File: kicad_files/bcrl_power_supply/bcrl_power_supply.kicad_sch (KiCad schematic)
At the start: 10 parts, among them J1 OSTVN02A150, J12 5034801600, J2 OSTVN02A150, J3 Conn_01x02

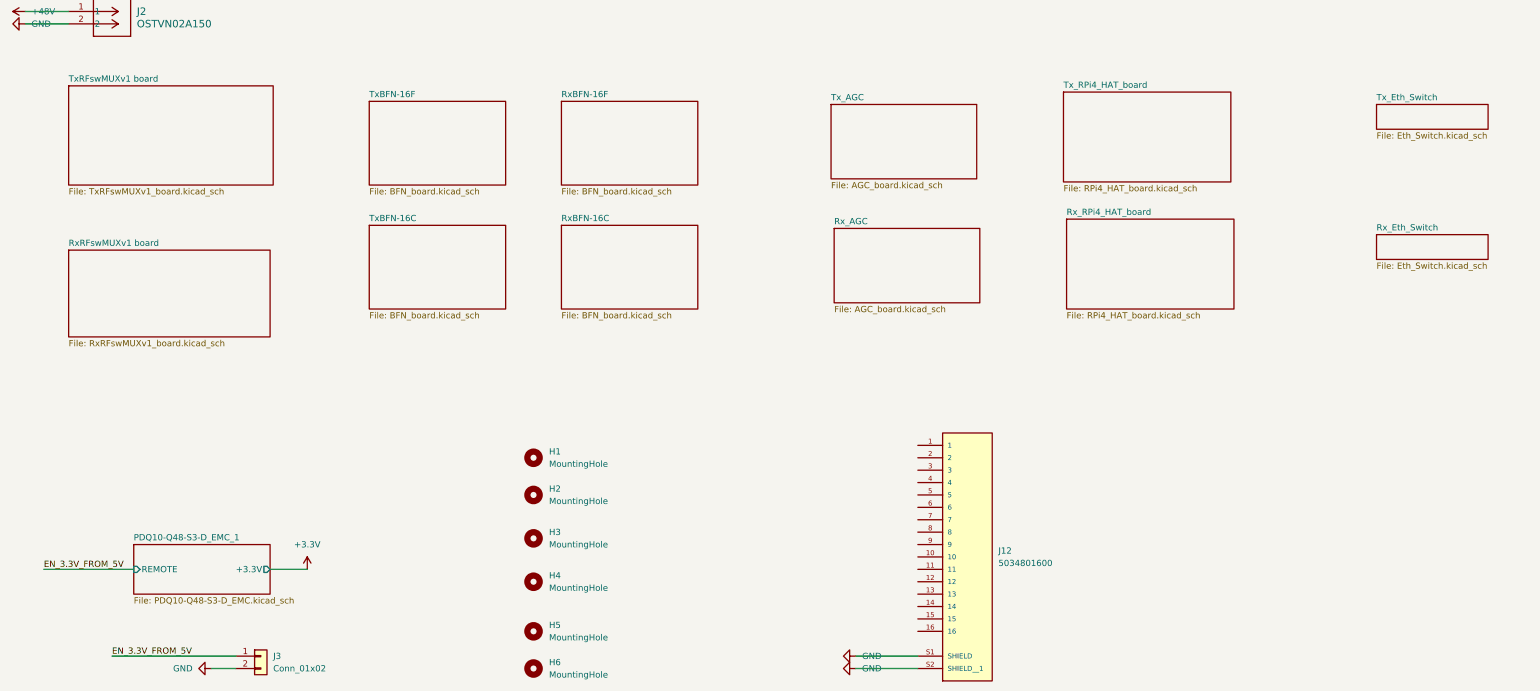
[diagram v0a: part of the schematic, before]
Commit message: almost done schematic
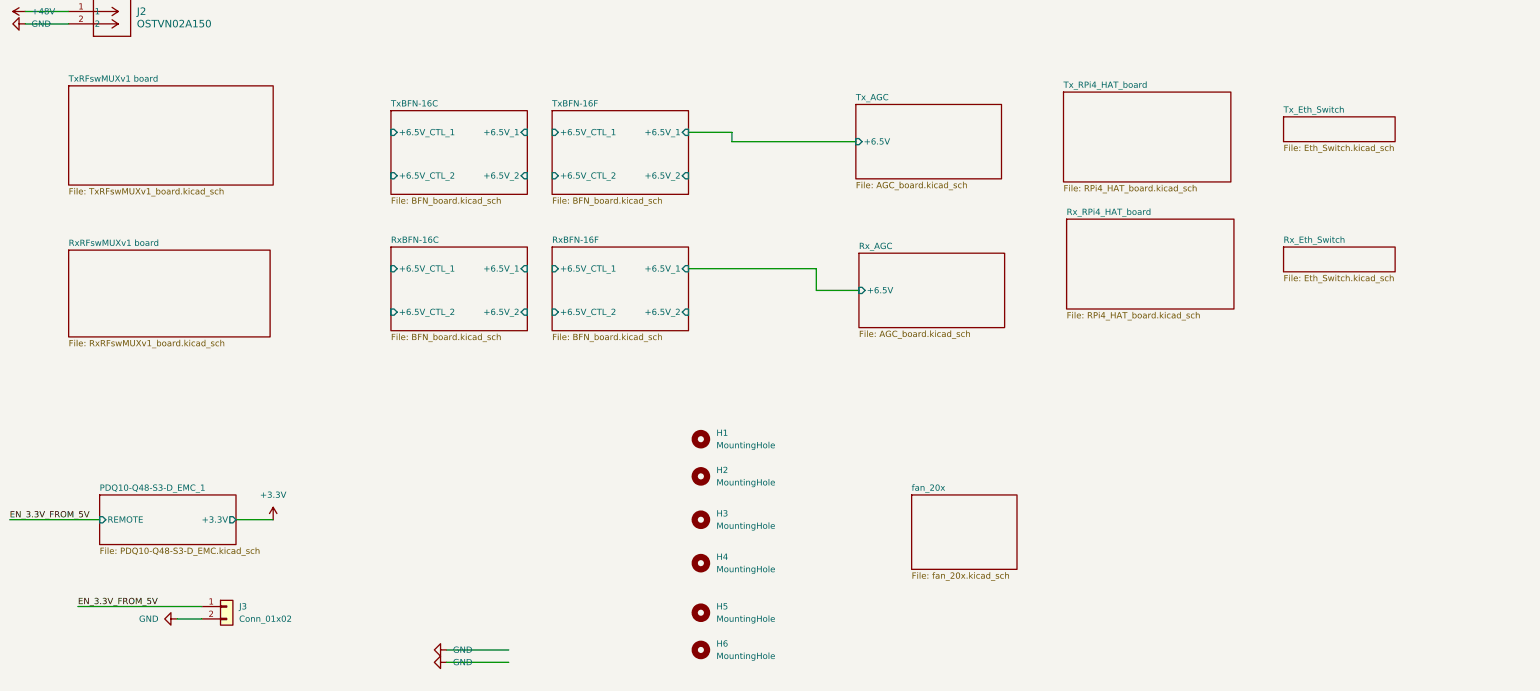
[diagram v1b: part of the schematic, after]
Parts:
- removed J12: 5034801600, BCRL_power_supply:MOLEX_5034801600, symbol BCRL_power_supply:5034801600
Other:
- added sheet fan_20x (fan_20x.kicad_sch)
- sheet RxBFN-16C ports: added +6.5V_1, +6.5V_2, +6.5V_CTL_1, +6.5V_CTL_2; removed none
- sheet RxBFN-16F ports: added +6.5V_1, +6.5V_2, +6.5V_CTL_1, +6.5V_CTL_2; removed none
- sheet Rx_AGC ports: added +6.5V; removed none
- sheet TxBFN-16C ports: added +6.5V_1, +6.5V_2, +6.5V_CTL_1, +6.5V_CTL_2; removed none
- sheet TxBFN-16F ports: added +6.5V_1, +6.5V_2, +6.5V_CTL_1, +6.5V_CTL_2; removed none
- sheet Tx_AGC ports: added +6.5V; removed none
- moved on the sheet: H1, H2, H3, H4, H5, H6, J3

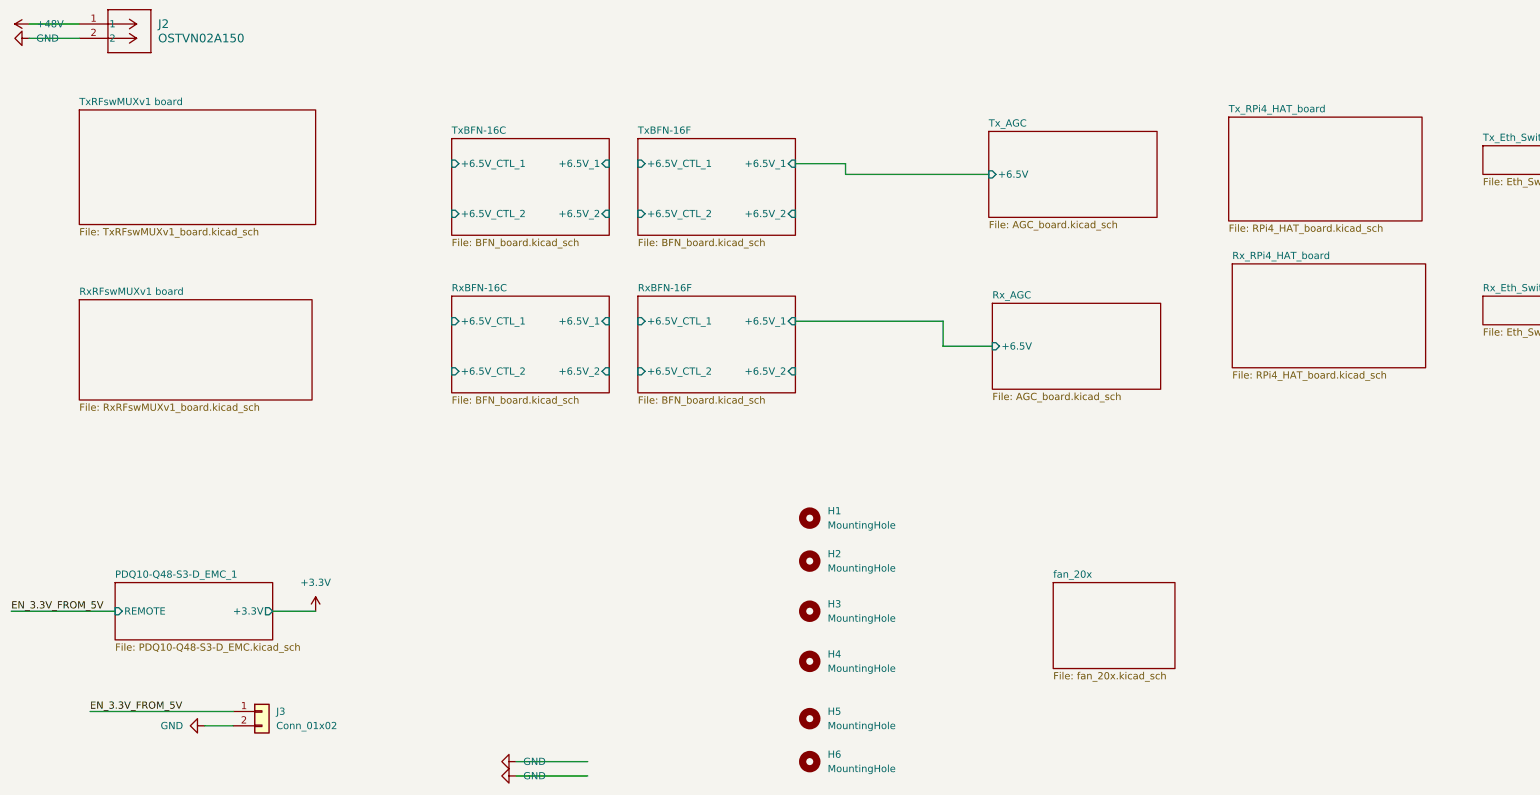
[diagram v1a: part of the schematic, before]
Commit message: schematic done
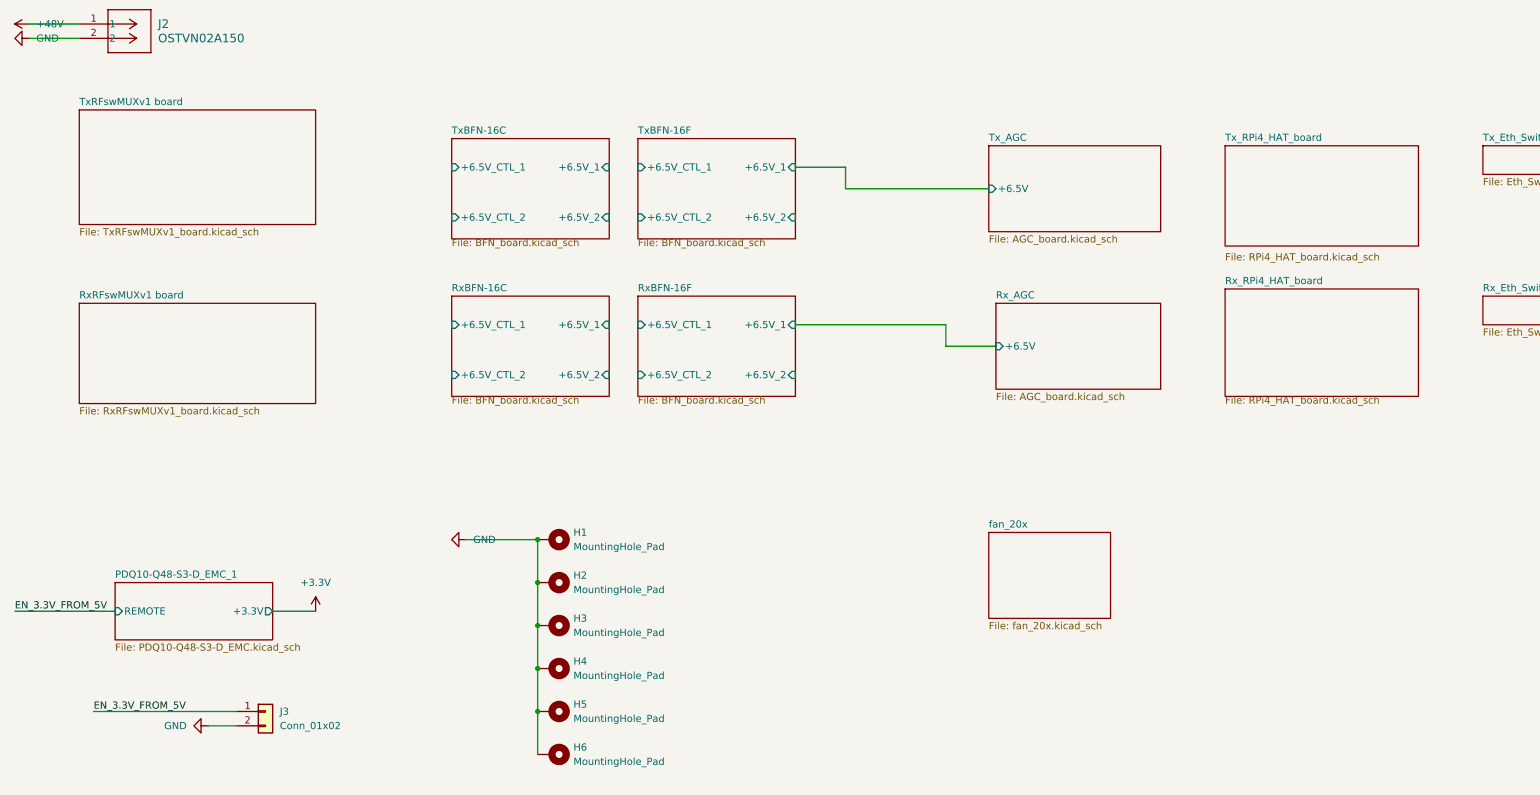
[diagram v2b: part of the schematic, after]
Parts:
- removed H1, H2, H3, H4, H5, H6: MountingHole, MountingHole:MountingHole_3.5mm_Pad, symbol Mechanical:MountingHole
- added H1, H2, H3, H4, H5, H6: MountingHole_Pad, MountingHole:MountingHole_3.5mm_Pad, symbol Mechanical:MountingHole_Pad
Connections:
- net GND: now also H1.1, H2.1, H3.1, H4.1, H5.1, H6.1
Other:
- moved on the sheet: J3

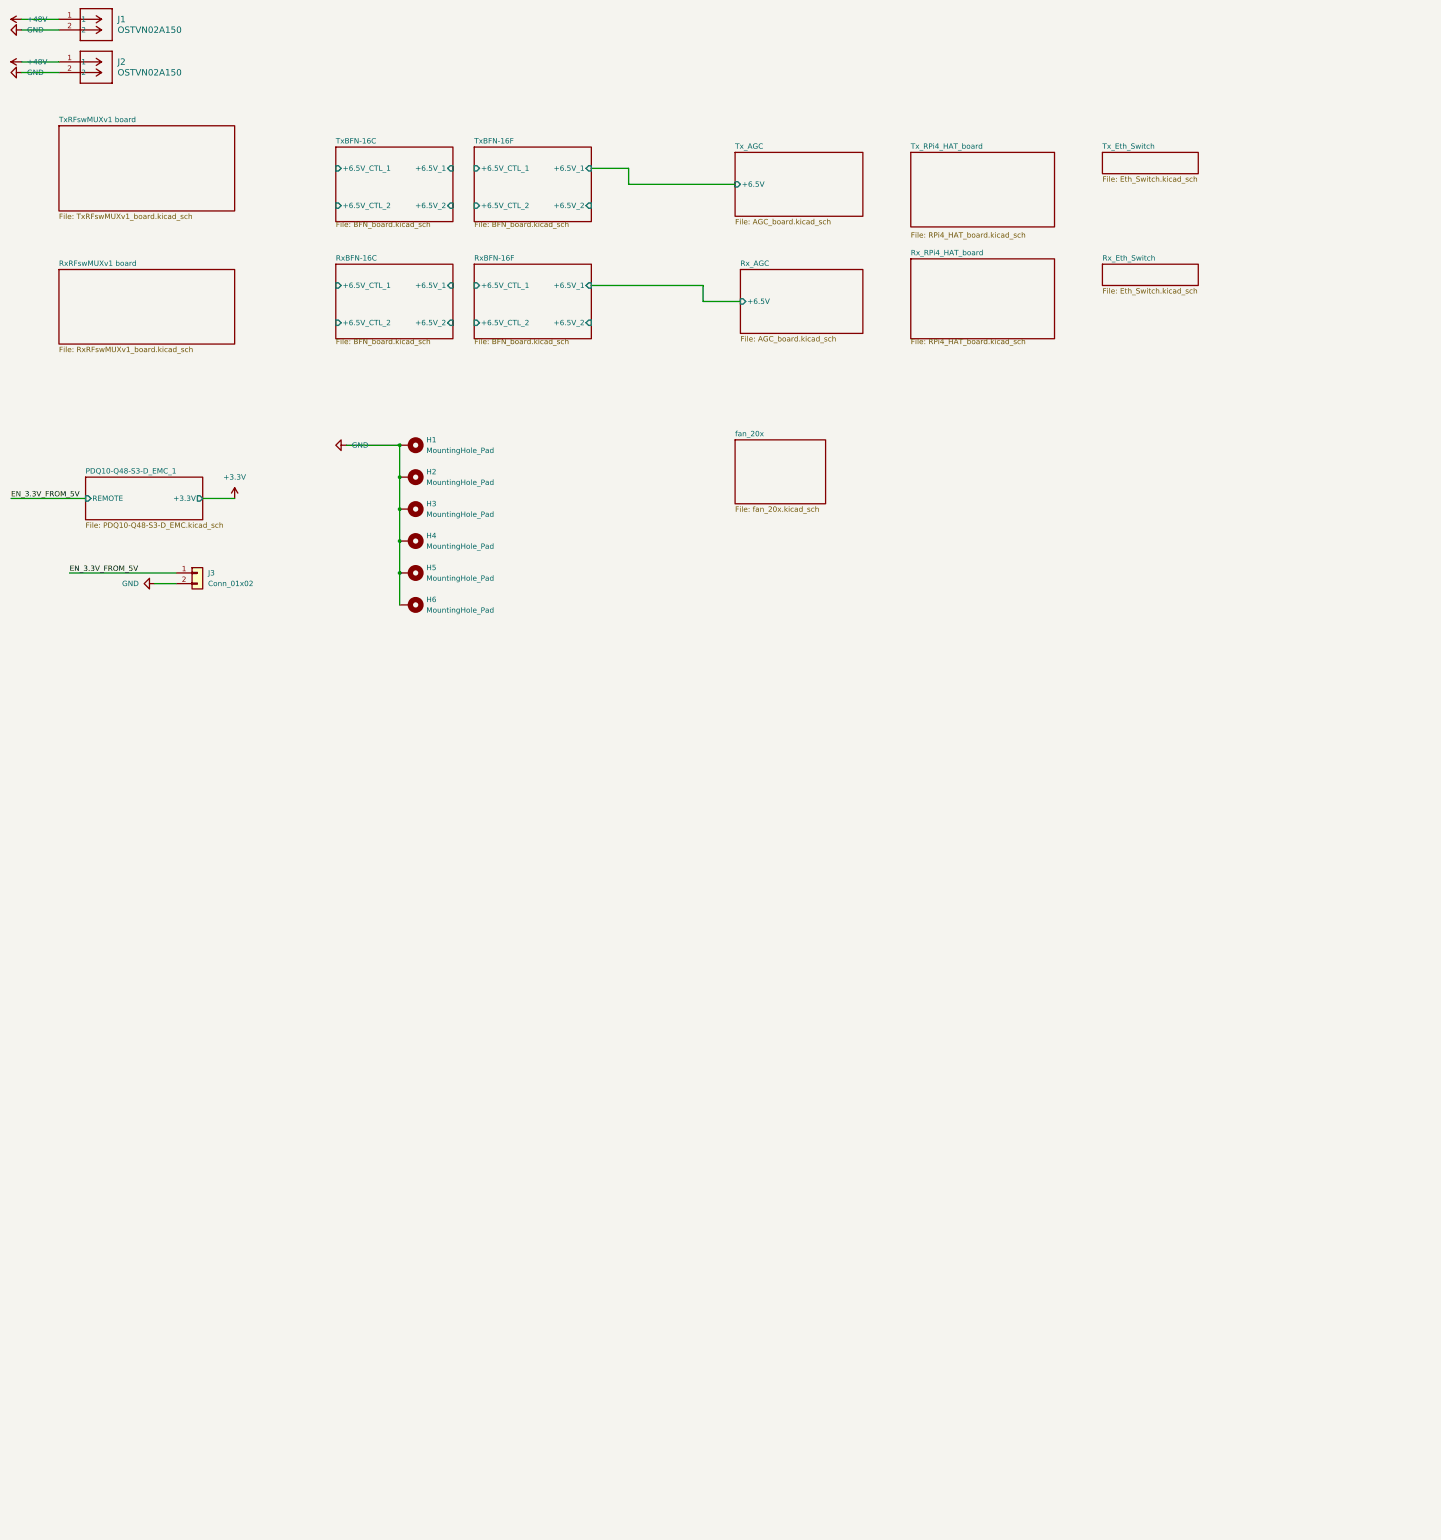
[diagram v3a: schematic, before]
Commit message: big reorg
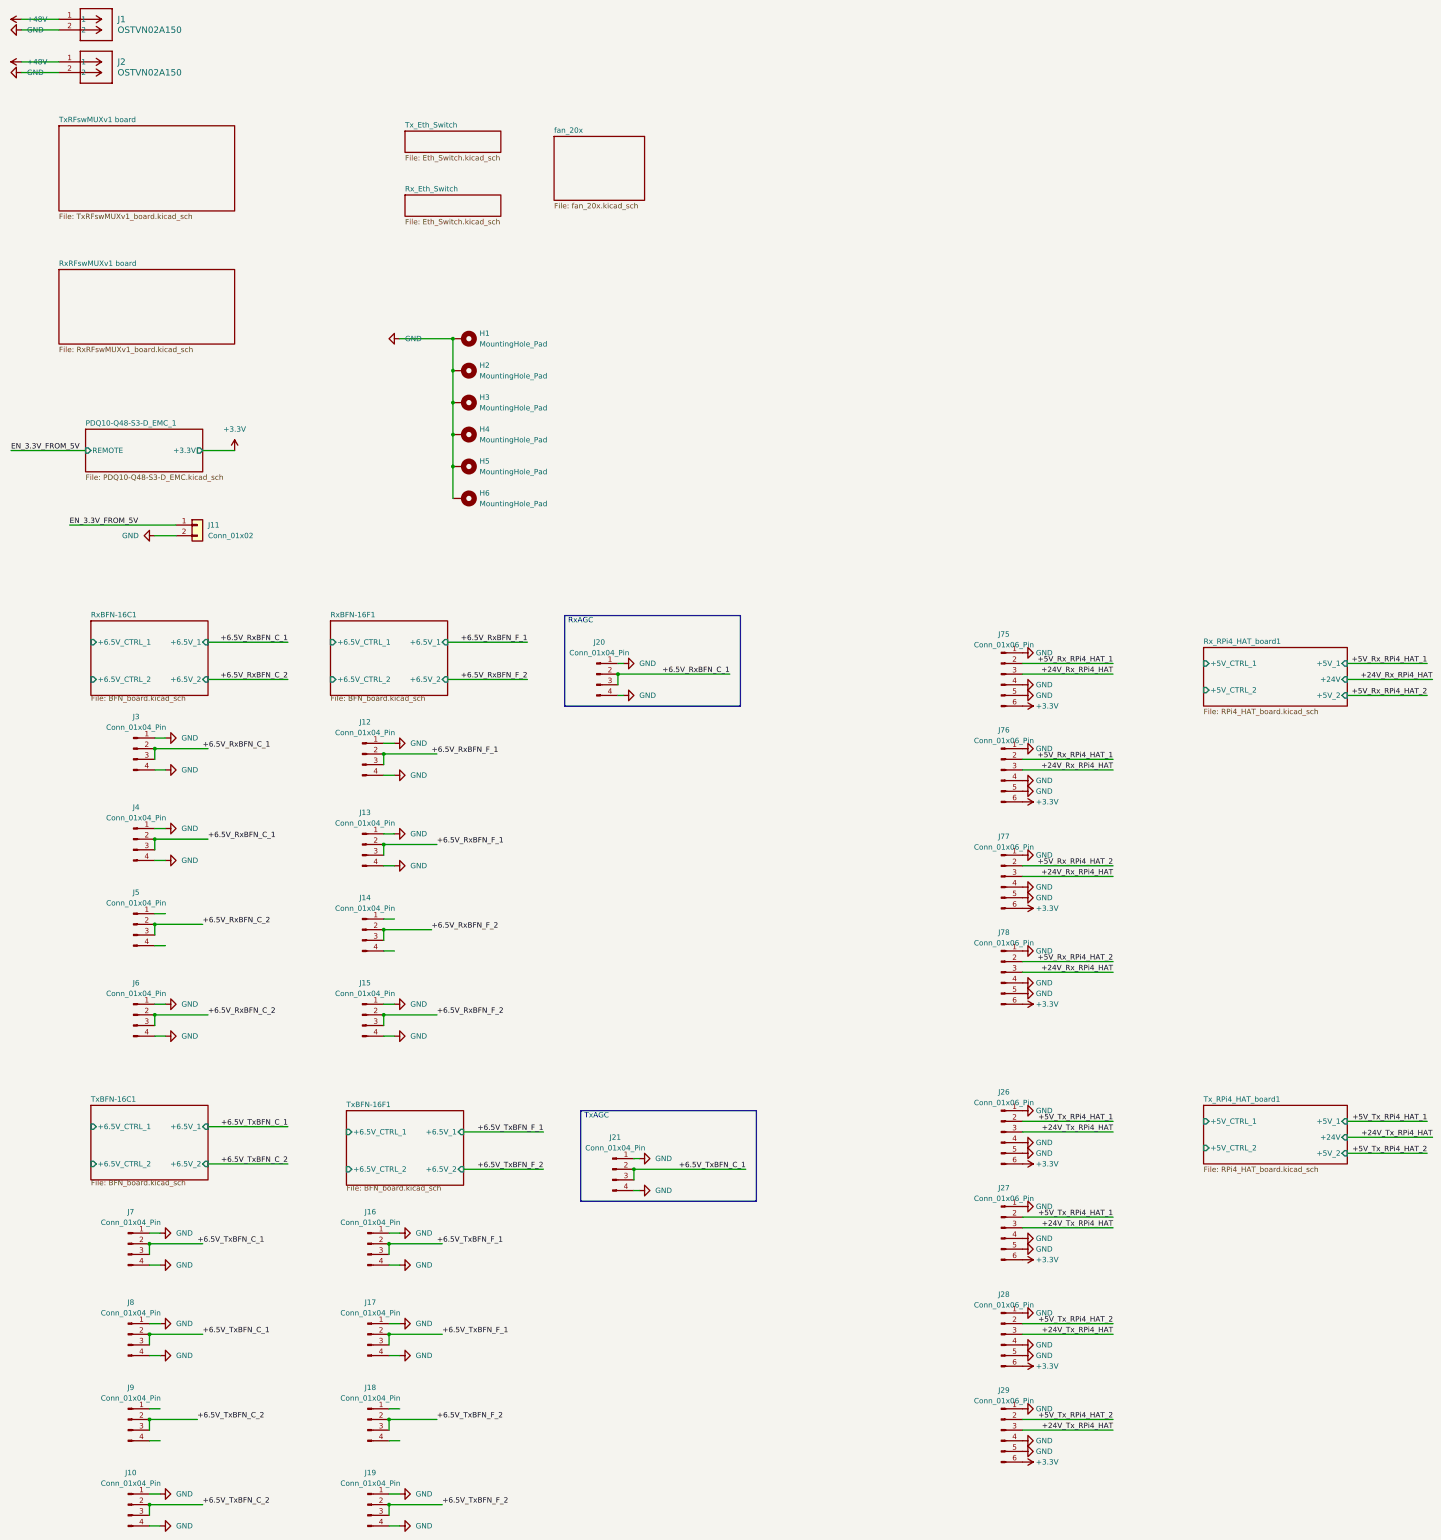
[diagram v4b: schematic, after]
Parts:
- added J10, J12, J13, J14, J15, J16, J17, J18, J19, J20, J21, J3, J4, J5, J6, J7, J8, J9: Conn_01x04_Pin, Connector_PinHeader_2.54mm:PinHeader_1x04_P2.54mm_Vertical, symbol Connector:Conn_01x04_Pin
- added J26, J27, J28, J29, J75, J76, J77, J78: Conn_01x06_Pin, Connector_PinHeader_2.54mm:PinHeader_1x06_P2.54mm_Vertical, symbol Connector:Conn_01x06_Pin
- renumbered J3 to J11
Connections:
- net +3.3V: now also J26.6 (Pin_6), J27.6 (Pin_6), J28.6 (Pin_6), J29.6 (Pin_6), J75.6 (Pin_6), J76.6 (Pin_6), J77.6 (Pin_6), J78.6 (Pin_6)
- net GND: now also J10.1 (Pin_1), J10.4 (Pin_4), J12.1 (Pin_1), J12.4 (Pin_4), J13.1 (Pin_1), J13.4 (Pin_4), J15.1 (Pin_1), J15.4 (Pin_4), J16.1 (Pin_1), J16.4 (Pin_4), J17.1 (Pin_1), J17.4 (Pin_4), J19.1 (Pin_1), J19.4 (Pin_4), J20.1 (Pin_1), J20.4 (Pin_4), J21.1 (Pin_1), J21.4 (Pin_4), J26.1 (Pin_1), J26.4 (Pin_4), J26.5 (Pin_5), J27.1 (Pin_1), J27.4 (Pin_4), J27.5 (Pin_5), J28.1 (Pin_1), J28.4 (Pin_4), J28.5 (Pin_5), J29.1 (Pin_1), J29.4 (Pin_4), J29.5 (Pin_5), J3.1 (Pin_1), J3.4 (Pin_4), J4.1 (Pin_1), J4.4 (Pin_4), J6.1 (Pin_1), J6.4 (Pin_4), J7.1 (Pin_1), J7.4 (Pin_4), J75.1 (Pin_1), J75.4 (Pin_4), J75.5 (Pin_5), J76.1 (Pin_1), J76.4 (Pin_4), J76.5 (Pin_5), J77.1 (Pin_1), J77.4 (Pin_4), J77.5 (Pin_5), J78.1 (Pin_1), J78.4 (Pin_4), J78.5 (Pin_5), J8.1 (Pin_1), J8.4 (Pin_4)
- new net +24V_Rx_RPi4_HAT: J75.3 (Pin_3), J76.3 (Pin_3), J77.3 (Pin_3), J78.3 (Pin_3)
- new net +24V_Tx_RPi4_HAT: J26.3 (Pin_3), J27.3 (Pin_3), J28.3 (Pin_3), J29.3 (Pin_3)
- new net +5V_Rx_RPi4_HAT_1: J75.2 (Pin_2), J76.2 (Pin_2)
- new net +5V_Rx_RPi4_HAT_2: J77.2 (Pin_2), J78.2 (Pin_2)
- new net +5V_Tx_RPi4_HAT_1: J26.2 (Pin_2), J27.2 (Pin_2)
- new net +5V_Tx_RPi4_HAT_2: J28.2 (Pin_2), J29.2 (Pin_2)
- new net +6.5V_RxBFN_C_1: J20.2 (Pin_2), J20.3 (Pin_3), J3.2 (Pin_2), J3.3 (Pin_3), J4.2 (Pin_2), J4.3 (Pin_3)
- new net +6.5V_RxBFN_C_2: J5.2 (Pin_2), J5.3 (Pin_3), J6.2 (Pin_2), J6.3 (Pin_3)
- new net +6.5V_RxBFN_F_1: J12.2 (Pin_2), J12.3 (Pin_3), J13.2 (Pin_2), J13.3 (Pin_3)
- new net +6.5V_RxBFN_F_2: J14.2 (Pin_2), J14.3 (Pin_3), J15.2 (Pin_2), J15.3 (Pin_3)
- new net +6.5V_TxBFN_C_1: J21.2 (Pin_2), J21.3 (Pin_3), J7.2 (Pin_2), J7.3 (Pin_3), J8.2 (Pin_2), J8.3 (Pin_3)
- new net +6.5V_TxBFN_C_2: J10.2 (Pin_2), J10.3 (Pin_3), J9.2 (Pin_2), J9.3 (Pin_3)
- new net +6.5V_TxBFN_F_1: J16.2 (Pin_2), J16.3 (Pin_3), J17.2 (Pin_2), J17.3 (Pin_3)
- new net +6.5V_TxBFN_F_2: J18.2 (Pin_2), J18.3 (Pin_3), J19.2 (Pin_2), J19.3 (Pin_3)
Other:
- removed sheet RxBFN-16C
- removed sheet RxBFN-16F
- removed sheet Rx_AGC
- removed sheet Rx_RPi4_HAT_board
- removed sheet TxBFN-16C
- removed sheet TxBFN-16F
- removed sheet Tx_AGC
- removed sheet Tx_RPi4_HAT_board
- added sheet RxBFN-16C1 (BFN_board.kicad_sch)
- added sheet RxBFN-16F1 (BFN_board.kicad_sch)
- added sheet Rx_RPi4_HAT_board1 (RPi4_HAT_board.kicad_sch)
- added sheet TxBFN-16C1 (BFN_board.kicad_sch)
- added sheet TxBFN-16F1 (BFN_board.kicad_sch)
- added sheet Tx_RPi4_HAT_board1 (RPi4_HAT_board.kicad_sch)
- note added: "RxAGC"
- note added: "TxAGC"
- moved on the sheet: H1, H2, H3, H4, H5, H6, J11
